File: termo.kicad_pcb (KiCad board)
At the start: 2 copper layers, 94 x 83.8 mm, 17 parts, among them J1 USB_A, J2 Conn_01x04_Female, J3 Conn_02x05_Odd_Even, U1 AMS1117, U2 ATmega324PA-AU, U3 HDC1080, Y1 Crystal

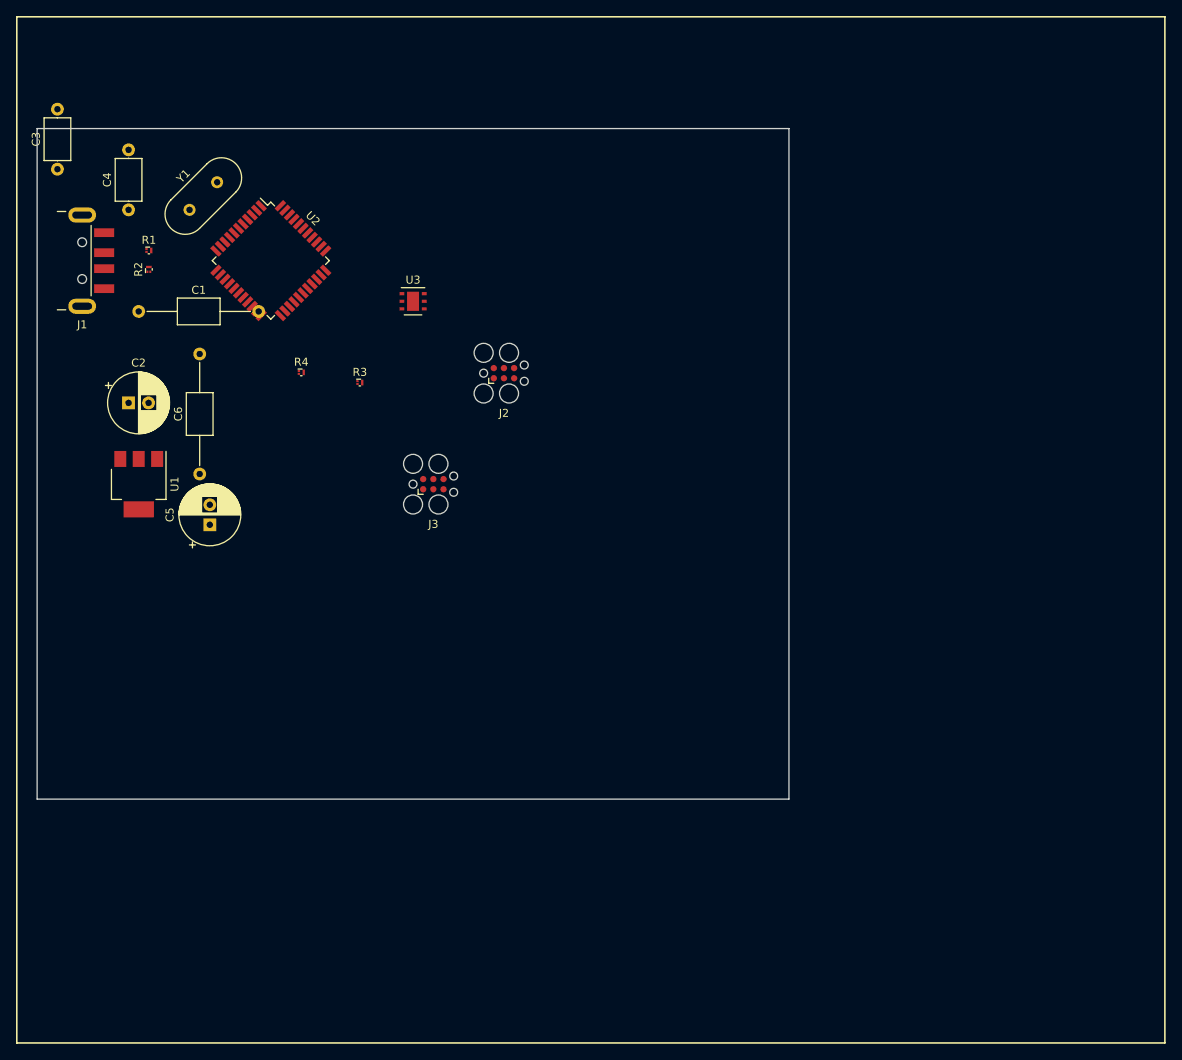
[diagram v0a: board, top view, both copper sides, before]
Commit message: Final layout
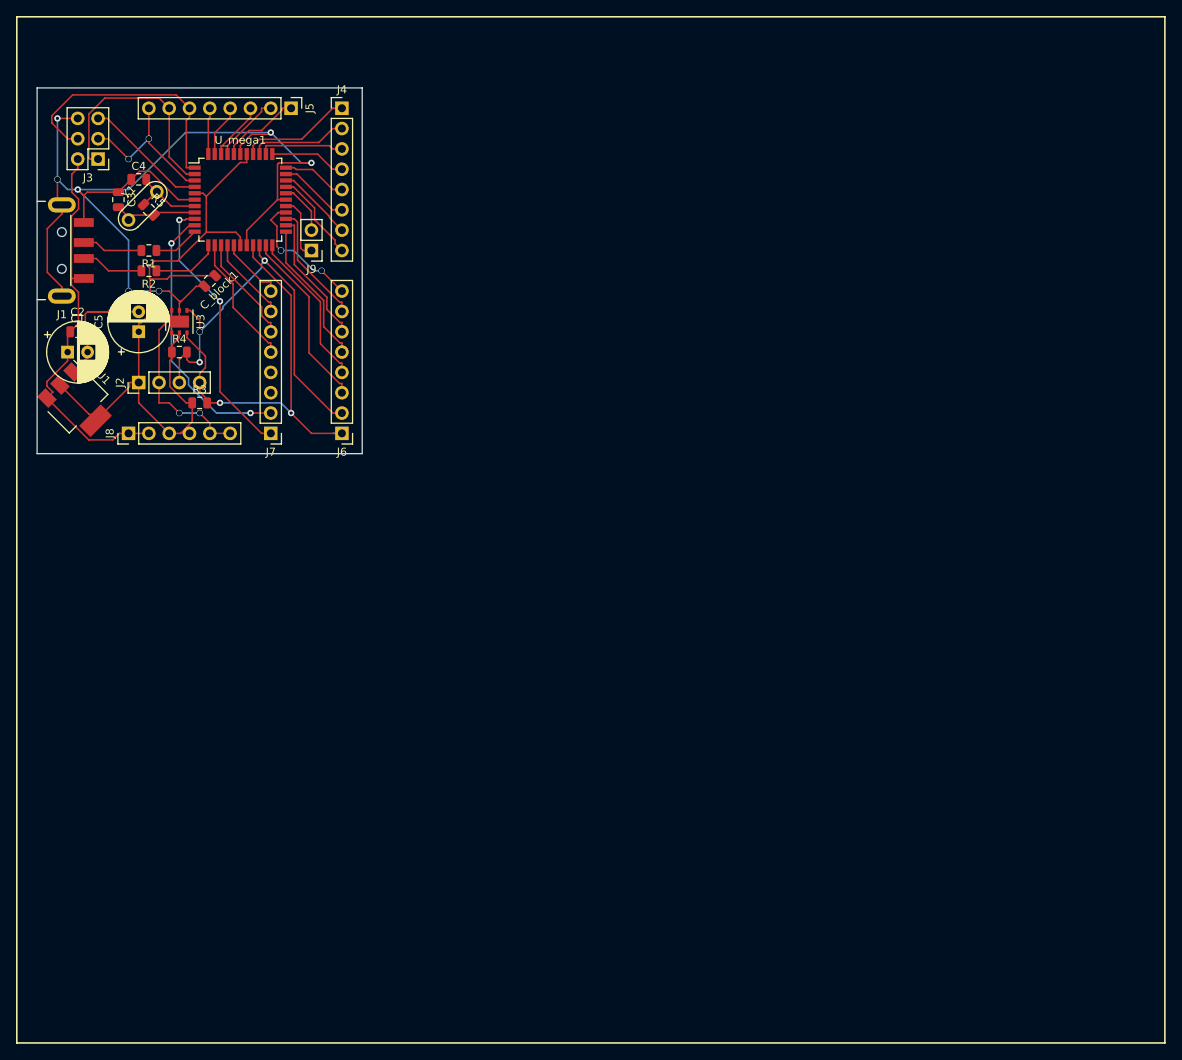
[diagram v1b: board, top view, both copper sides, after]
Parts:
- removed C6: C, Capacitor_THT:C_Axial_L5.1mm_D3.1mm_P15.00mm_Horizontal
- removed U2: ATmega324PA-AU, Package_QFP:TQFP-44_10x10mm_P0.8mm
- added C_block1: C, Capacitor_SMD:C_0805_2012Metric, F.Cu at (39.4, 45.7)
- added J4: PA, Connector_PinHeader_2.54mm:PinHeader_1x08_P2.54mm_Vertical, F.Cu at (55.9, 24.1)
- added J5: PB, Connector_PinHeader_2.54mm:PinHeader_1x08_P2.54mm_Vertical, F.Cu at (49.5, 24.1)
- added J6: PC, Connector_PinHeader_2.54mm:PinHeader_1x08_P2.54mm_Vertical, F.Cu at (55.9, 64.8)
- added J7: PD, Connector_PinHeader_2.54mm:PinHeader_1x08_P2.54mm_Vertical, F.Cu at (47.0, 64.8)
- added J8: PWR, Connector_PinHeader_2.54mm:PinHeader_1x06_P2.54mm_Vertical, F.Cu at (29.2, 64.8)
- added J9: PA, Connector_PinHeader_2.54mm:PinHeader_1x02_P2.54mm_Vertical, F.Cu at (52.1, 41.9)
- added R5: R, Resistor_SMD:R_0805_2012Metric, F.Cu at (31.8, 36.8)
- added U_mega1: ATmega16-16AU, Package_QFP:TQFP-44_10x10mm_P0.8mm, F.Cu at (43.2, 35.6)
- C1: footprint Capacitor_THT:C_Axial_L5.1mm_D3.1mm_P15.00mm_Horizontal -> Capacitor_SMD:C_0805_2012Metric
- C3, C4: footprint Capacitor_THT:C_Axial_L5.1mm_D3.1mm_P7.50mm_Horizontal -> Capacitor_SMD:C_0805_2012Metric
- J2: footprint Connector:Tag-Connect_TC2030-IDC-FP_2x03_P1.27mm_Vertical -> Connector_PinHeader_2.54mm:PinHeader_1x04_P2.54mm_Vertical
- J3: value Conn_02x05_Odd_Even -> ISP; footprint Connector:Tag-Connect_TC2030-IDC-FP_2x03_P1.27mm_Vertical -> Connector_PinHeader_2.54mm:PinHeader_2x03_P2.54mm_Vertical
- R1, R2, R3, R4: footprint Package_SON:ROHM_VML0806 -> Resistor_SMD:R_0805_2012Metric
- Y1: footprint Crystal:Crystal_HC49-4H_Vertical -> Crystal:Resonator-2Pin_W7.0mm_H2.5mm
- moved J3 58.4 mm to (25.4, 30.5), turned to 180 degrees
- moved J2 45.7 mm to (30.5, 58.4), turned to 90 degrees
- moved U3 29.3 mm to (35.6, 50.8), turned to 270 degrees
- moved C5 25.7 mm to (30.5, 52.1)
- moved R3 20.2 mm to (38.1, 61.0)
- moved R4 15.5 mm to (35.6, 54.6)
- moved U1 12.7 mm to (22.9, 61.0), turned to 315 degrees
- moved C2 9.92 mm to (21.6, 54.6)
- moved C3 8.52 mm to (27.9, 35.6), turned to 270 degrees
- moved C1 8.03 mm to (22.9, 52.1)
- moved Y1 7.73 mm to (29.2, 38.1)
- moved C4 4.02 mm to (30.5, 33.0), turned to 0 degrees
- moved J1 2.84 mm to (14.0, 41.9)
- moved R2 0.18 mm to (31.8, 44.5), turned to 180 degrees
- turned R1 to 180 degrees
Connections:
- C3 pad 1: Net-(C3-Pad1) -> GNDD
- C4 pad 1: Net-(C3-Pad1) -> GNDD
- J3 pad 1: mosi -> miso
- J3 pad 3: (no net) -> sck
- J3 pad 4: GNDD -> mosi
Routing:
- net GNDD: track 0.00 -> 181.5 mm, vias 0 -> 9
- net +3V3: track 0.00 -> 92.5 mm
- net scl: track 0.00 -> 52.9 mm, vias 0 -> 2
- net sda: track 0.00 -> 52.4 mm, vias 0 -> 3
- net +5V: track 0.00 -> 50.3 mm
- net Net-(J7-Pad2): track 0.00 -> 34.4 mm, vias 0 -> 2
- net Net-(J7-Pad1): track 0.00 -> 34.1 mm, vias 0 -> 2
- net mosi: track 0.00 -> 32.6 mm
- net miso: track 0.00 -> 28.3 mm
- net Net-(J6-Pad3): track 0.00 -> 22.5 mm
- net sck: track 0.00 -> 20.5 mm, vias 0 -> 2
- net Net-(J6-Pad4): track 0.00 -> 19.6 mm
- net Net-(J6-Pad5): track 0.00 -> 18.1 mm
- net Net-(J6-Pad6): track 0.00 -> 17.0 mm
- net Net-(J7-Pad5): track 0.00 -> 16.4 mm
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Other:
- board size 94 x 83.8 mm -> 40.6 x 45.7 mm
- net class Default: trace_width 0.4 -> 0.2; via_drill 0.4 -> 0.7
- rule trace_min: 0.4 -> 0.2
- rule via_min_drill: 0.4 -> 0.6
- rule via_min_size: 0.4 -> 0.7
